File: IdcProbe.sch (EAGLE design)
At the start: 66 parts, among them IC1 TL074D, P1 BANANA_SOCKETVERTICAL, P2 BANANA_SOCKETVERTICAL, U1 TPS65131RGET, X3 R141426

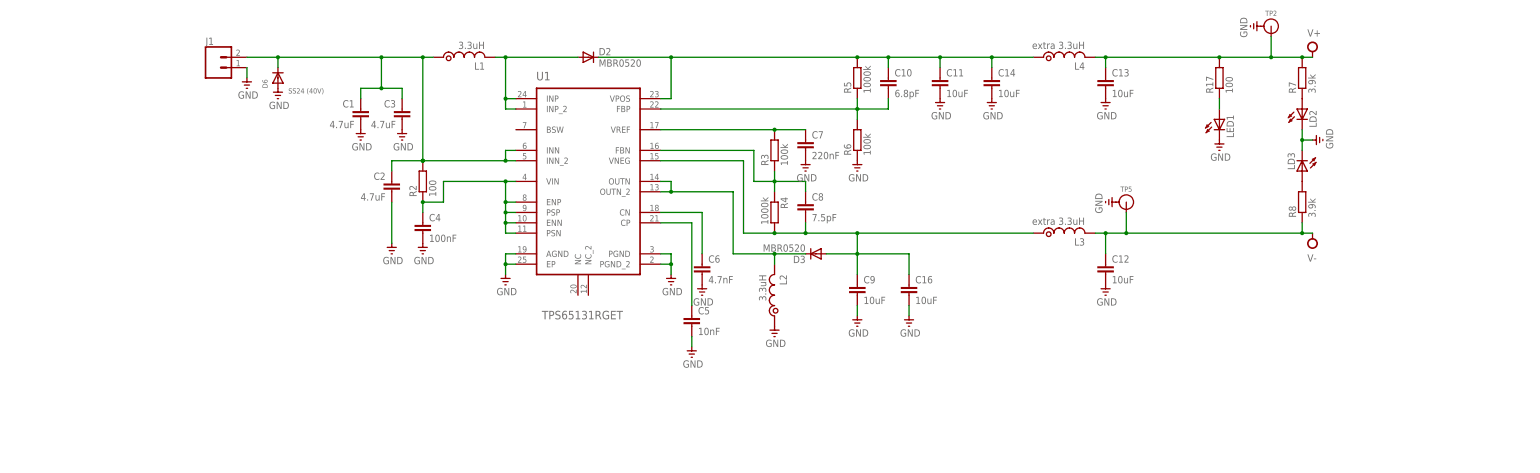
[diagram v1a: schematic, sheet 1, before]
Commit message: Update smps
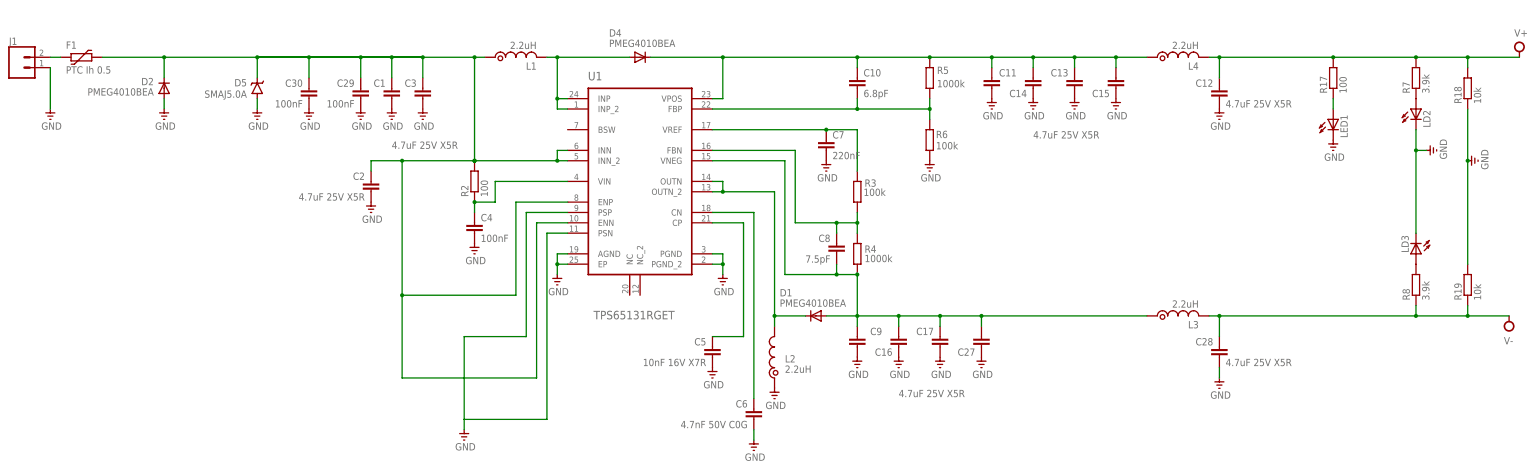
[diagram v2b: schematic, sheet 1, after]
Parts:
- removed D3: MBR0520, diode:DIODE-SOD123
- removed D6: SS24 (40V), microbuilder:DIODESMA
- removed TP2, TP5: TESTPOINT_GND, Jeroen:TESTPOINT_GND
- added C15, C17, C27, C28: 4.7uF 25V X5R, rcl:C-EUC0805
- added C29, C30: 100nF, rcl:C-EUC0805
- added D1, D4: PMEG4010BEA, diode:DIODE-SOD323-R
- added D5: SMAJ5.0A, Jeroen:SMAJ13A-TR
- added F1: PTC Ih 0.5, dp_devices:FUSE_PTC-0805
- added R18, R19: 10k, rcl:R-EU_R0805I
- C1, C2, C3: value 4.7uF -> 4.7uF 25V X5R
- C11, C12, C13, C14, C16, C9: value 10uF -> 4.7uF 25V X5R; device rcl:C-EUC1206 -> rcl:C-EUC0805
- C5: value 10nF -> 10nF 16V X7R
- C6: value 4.7nF -> 4.7nF 50V C0G
- D2: value MBR0520 -> PMEG4010BEA; device diode:DIODE-SOD123 -> diode:DIODE-SOD323-R
- L1, L2: value 3.3uH -> 2.2uH
- L3, L4: value extra 3.3uH -> 2.2uH
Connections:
- new net N$21: F1.1, J1.2
- net GND: now also C15.2, C17.2, C27.2, C28.2, C29.2, C30.2, D2.A, D5.A, R18.1, R19.2, U1.PSN, U1.PSP; no longer D6.A, TP2.P$2, TP5.P$2
- net INP: now also D4.A; no longer D2.A
- net OUTN: now also D1.C; no longer D3.C
- net RV+: now also C13.1, C15.1, D4.C; no longer D2.C
- net RV-: now also C17.1, C27.1, D1.A; no longer D3.A
- net V+: now also C12.1, R18.2; no longer C13.1, TP2.P$1
- net V-: now also C28.1, R19.1; no longer C12.1, TP5.P$1
- net VI: now also C29.1, C30.1, D2.C, D5.C, F1.2, U1.ENN, U1.ENP; no longer D6.C, J1.2
- net VIN: no longer U1.ENN, U1.ENP, U1.PSN, U1.PSP
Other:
- note added: "Base load"
- note added: "Booster"
- note added: "Disable power save mode"
- note added: "Enable Negative"
- note added: "Enable Positive"
- note added: "Extra filter"
- note added: "Inverter"
- note added: "Overvoltage"
- note added: "Polyfuse"
- note added: "Reverse polarity"
- note removed: "should be 22uF"
- moved on the sheet: C1, C10, C11, C12, C13, C14, C16, C2, C3, C4, C5, C6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
